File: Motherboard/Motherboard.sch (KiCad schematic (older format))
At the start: 116 parts, among them J1 Jack-DC_18v, J2 65SIB_Connector, J3 DB9_Header, J4 GPIO_Connector, J5 Expansion_Connector, J6 Expansion_Connector, J7 Expansion_Connector, J8 Expansion_Connector, J9 Expansion_Connector, P1 POWER TERMINAL, Q1 2N3055, Q2 TIC106, SW1 POWER SELECT, SW2 FUSE RESET, SW3 PROCESSOR RESET, U1 LM7812_TO220, U10 74HCT541, U11 28C256, U12 LM386, U13 LM7912_TO220, U14 74HCT00, U15 74HCT04, U16 74HCT574, U17 74HCT574, U18 74LS08, U19 28C256, U2 LM7805_TO220, U20 74LS138, U21 WD65C02, U22 74LS138, U23 74HCT04, U24 74HC74, U25 W65C51N, U26 NE555P, U27 WD65C22, U28 74LS138, U29 MAX235, U3 74LS08, U30 74LS138, U31 74HCT04, U32 74HCT04, U33 WD65C22, U34 74LS138, U35 74LS21, U36 74HCT04, U37 74LS21, U38 74HCT04, U39 74LS21, U4 74LS148, U40 74LS08, U41 74LS138, U42 74LS08, U43 74HCT04, U5 74LS85, U6 74HCT00, U7 74HCT04, U8 74LS08, U9 HM62256BLP, X1 ACO-8MHz, X2 ACO-1.8432MHz

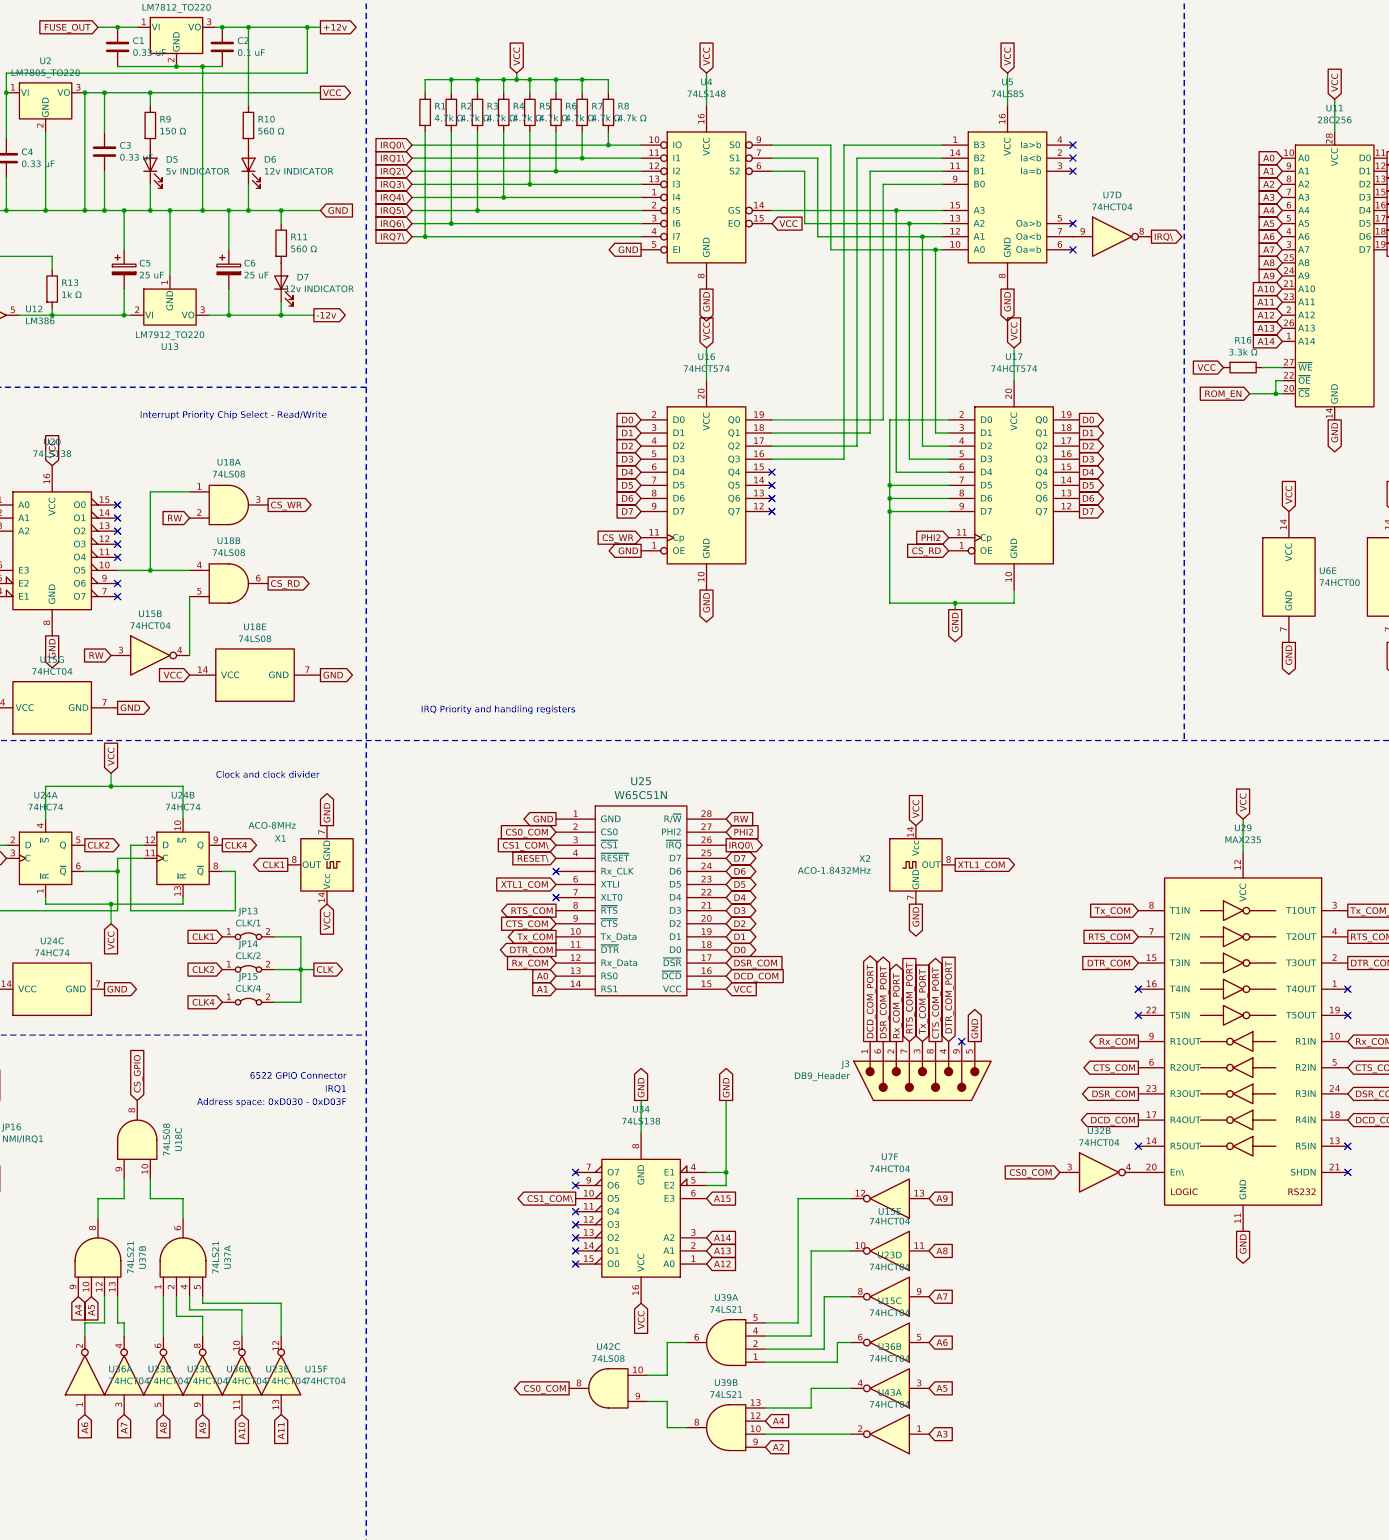
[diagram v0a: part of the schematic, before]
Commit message: Completed version 2 schematic...
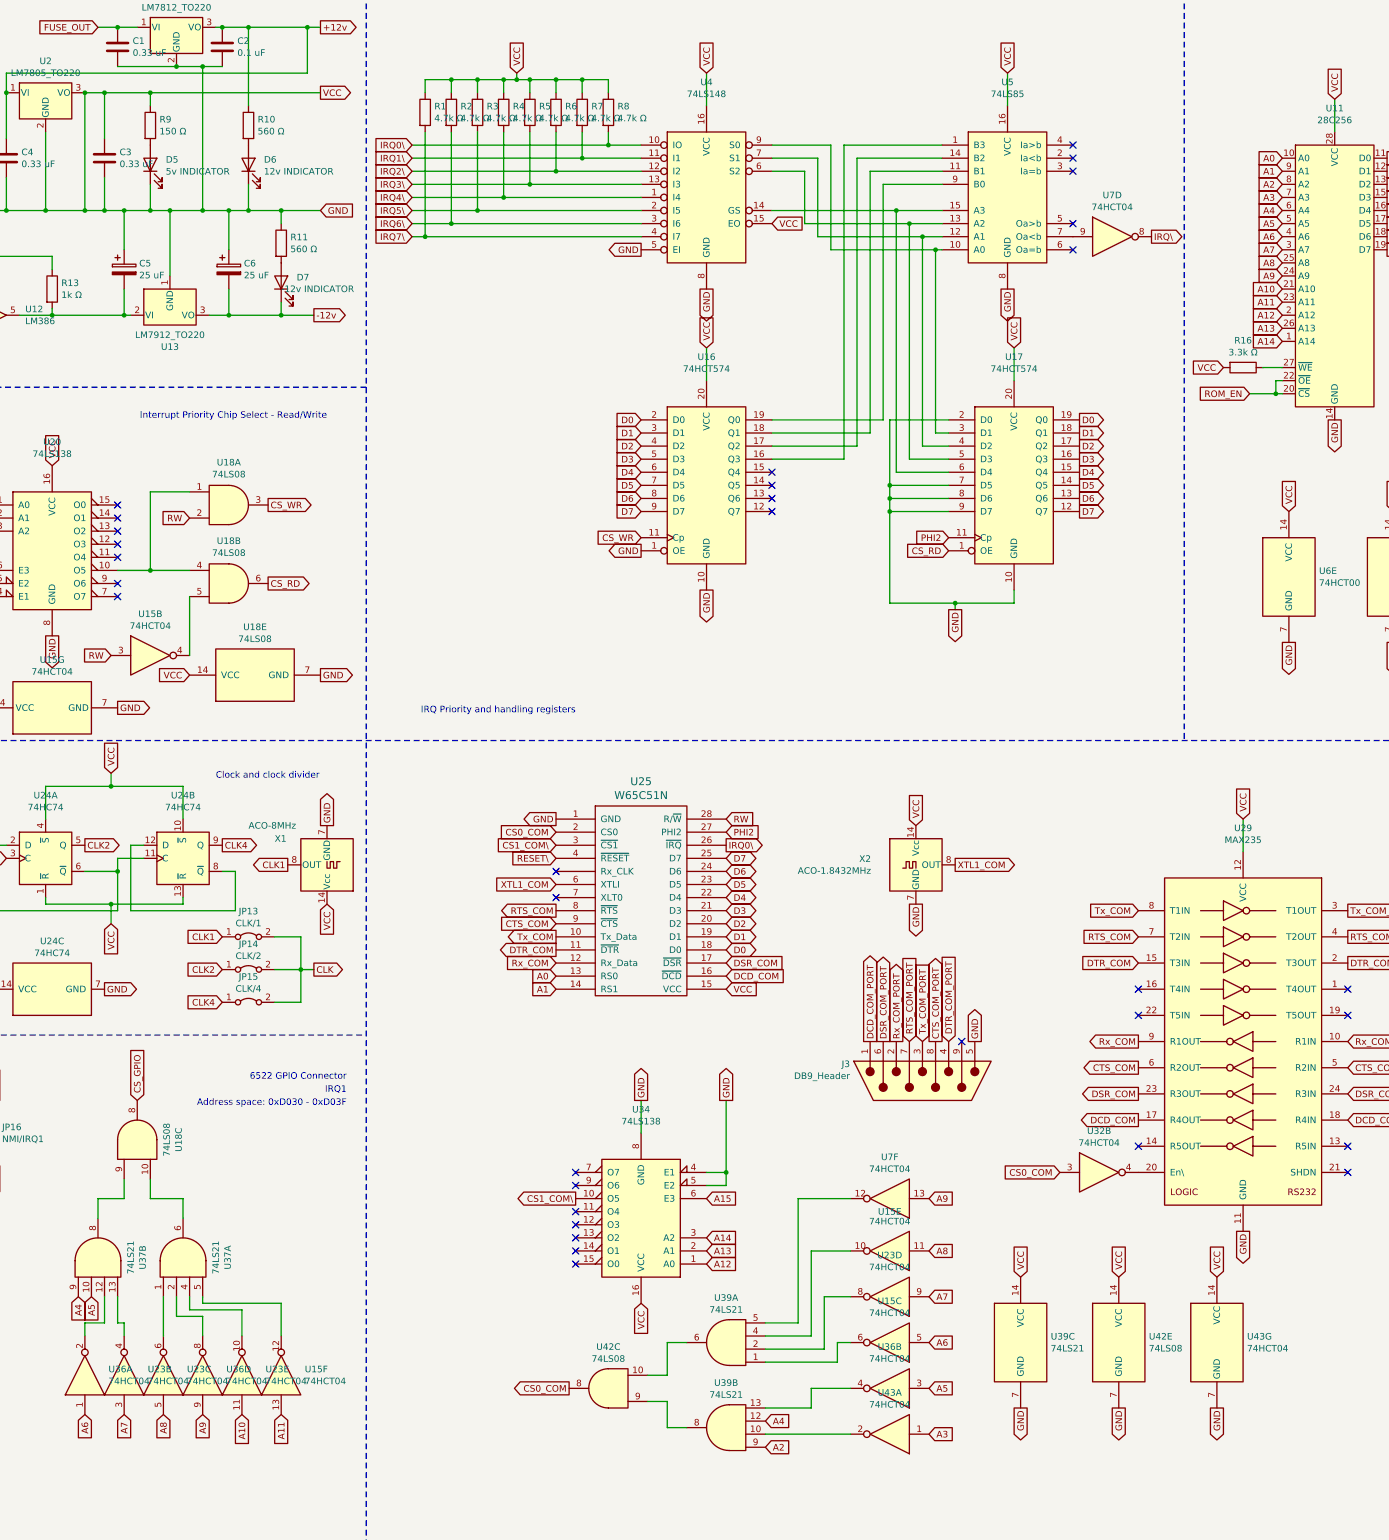
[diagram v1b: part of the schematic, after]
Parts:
- added unit 3 of U39
- added unit 5 of U42
- added unit 7 of U43
- U27: footprint Package_DIP:DIP-28_W15.24mm_Socket_LongPads -> Package_DIP:DIP-40_W15.24mm_Socket_LongPads
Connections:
- net GND: now also U39.14 (VCC), U39.7 (GND), U42.14 (VCC), U42.7 (GND), U43.14 (VCC), U43.7 (GND)
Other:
- moved on the sheet: C3
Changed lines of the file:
@@
 L Device:C C3
 U 1 1 61918BA3
-P 6700 2650
-F 0 "C3" H 6815 2696 50  0000 L CNN
-F 1 "0.33 uF" H 6815 2605 50  0000 L CNN
-F 2 "Capacitor_THT:C_Disc_D3.0mm_W1.6mm_P2.50mm" H 6738 2500 50  0001 C CNN
-F 3 "~" H 6700 2650 50  0001 C CNN
-	1    6700 2650
+P 6700 2700
+F 0 "C3" H 6815 2746 50  0000 L CNN
+F 1 "0.33 uF" H 6815 2655 50  0000 L CNN
+F 2 "Capacitor_THT:C_Disc_D3.0mm_W1.6mm_P2.50mm" H 6738 2550 50  0001 C CNN
+F 3 "~" H 6700 2700 50  0001 C CNN
+	1    6700 2700
 	1    0    0    -1
 $EndComp
 Wire Wire Line
-	6700 2800 6700 3100
-Wire Wire Line
-	6700 2500 6700 2200
-Wire Wire Line
 	2350 3100 3750 3100
 $Comp
@@
 Wire Wire Line
 	7050 2900 7050 3100
-Connection ~ 6700 3100
-Wire Wire Line
-	6700 2200 7050 2200
 Wire Wire Line
 	7050 2200 7050 2300
@@
 $EndComp
 Wire Wire Line
-	6550 2200 6700 2200
-Connection ~ 6700 2200
-Wire Wire Line
 	6250 2500 6250 3100
 $Comp
@@
 	7800 1700 8250 1700
 Connection ~ 6550 3100
-Wire Wire Line
-	6550 3100 6700 3100
 Connection ~ 6550 2200
 Wire Wire Line
@@
 $EndComp
 Wire Wire Line
-	6700 3100 6850 3100
-Wire Wire Line
 	7450 3100 7650 3100
 Wire Wire Line
@@
 F 0 "U27" H 24350 7413 60  0000 C CNN
 F 1 "WD65C22" H 24350 7519 60  0000 C CNN
-F 2 "Package_DIP:DIP-28_W15.24mm_Socket_LongPads" H 23850 8850 60  0001 C CNN
+F 2 "Package_DIP:DIP-40_W15.24mm_Socket_LongPads" H 23850 8850 60  0001 C CNN
 F 3 "" H 23850 8850 60  0000 C CNN
 	1    24350 8650
@@
 GND
 NoConn ~ 16200 10450
+$Comp
+L 74xx:74LS21 U39
+U 3 1 626DCCF3
+P 13700 11750
+F 0 "U39" H 13930 11796 50  0000 L CNN
+F 1 "74LS21" H 13930 11705 50  0000 L CNN
+F 2 "Package_DIP:DIP-14_W7.62mm_Socket_LongPads" H 13700 11750 50  0001 C CNN
+F 3 "http://www.ti.com/lit/gpn/sn74LS21" H 13700 11750 50  0001 C CNN
+	3    13700 11750
+	1    0    0    -1
+$EndComp
+Text GLabel 13700 11250 1    50   Input ~ 0
+VCC
+Text GLabel 13700 12250 3    50   Output ~ 0
+GND
+$Comp
+L 74xx:74LS08 U42
+U 5 1 626EAF96
+P 14450 11750
+F 0 "U42" H 14680 11796 50  0000 L CNN
+F 1 "74LS08" H 14680 11705 50  0000 L CNN
+F 2 "Package_DIP:DIP-14_W7.62mm_Socket_LongPads" H 14450 11750 50  0001 C CNN
+F 3 "http://www.ti.com/lit/gpn/sn74LS08" H 14450 11750 50  0001 C CNN
+	5    14450 11750
+	1    0    0    -1
+$EndComp
+Text GLabel 14450 11250 1    50   Input ~ 0
+VCC
+Text GLabel 14450 12250 3    50   Output ~ 0
+GND
+$Comp
+L 74xx:74HCT04 U43
+U 7 1 626F5FEB
+P 15200 11750
+F 0 "U43" H 15430 11796 50  0000 L CNN
+F 1 "74HCT04" H 15430 11705 50  0000 L CNN
+F 2 "Package_DIP:DIP-14_W7.62mm_Socket_LongPads" H 15200 11750 50  0001 C CNN
+F 3 "https://assets.nexperia.com/documents/data-sheet/74HC_HCT04.pdf" H 15200 11750 50  0001 C CNN
+	7    15200 11750
+	1    0    0    -1
+$EndComp
+Text GLabel 15200 11250 1    50   Input ~ 0
+VCC
+Text GLabel 15200 12250 3    50   Output ~ 0
+GND
+Wire Wire Line
+	6550 2200 6700 2200
+Wire Wire Line
+	6550 3100 6700 3100
+Wire Wire Line
+	6700 2850 6700 3100
+Connection ~ 6700 3100
+Wire Wire Line
+	6700 3100 6850 3100
+Wire Wire Line
+	6700 2550 6700 2200
+Connection ~ 6700 2200
+Wire Wire Line
+	6700 2200 7050 2200
 $EndSCHEMATC

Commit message: Various bug fixes and more traces added....
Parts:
- removed U20, U34, U41: 74LS138, Package_DIP:DIP-16_W7.62mm_Socket_LongPads, symbol 74xx:74LS138
- SW1: value POWER SELECT -> Barrel Jack / Mains
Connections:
- net 65SIB_CS2\ is gone; now on net DEV_CS\: U27.23 (~CS2), U28.10 (O5), U30.5 (E2)
- net CS1_COM\ is gone; now on net DEV_CS\: U25.3 (~CS1)
- net NMI\: no longer J5.28 (Pin_28), J6.28 (Pin_28), J7.28 (Pin_28), J8.28 (Pin_28), J9.28 (Pin_28)
- net DEV_CS\: now reaches U18.1, U18.4
- net DEV_CS\: now also U33.23 (~CS2)
- no-connect marks 68 -> 52
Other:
- moved on the sheet: U28
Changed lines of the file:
@@
 Wire Wire Line
 	2900 5650 3850 5650
-$Comp
-L 74xx:74LS138 U20
-U 1 1 6193D1D9
-P 6300 5650
-F 0 "U20" H 6300 6431 50  0000 C CNN
-F 1 "74LS138" H 6300 6340 50  0000 C CNN
-F 2 "Package_DIP:DIP-16_W7.62mm_Socket_LongPads" H 6300 5650 50  0001 C CNN
-F 3 "http://www.ti.com/lit/gpn/sn74LS138" H 6300 5650 50  0001 C CNN
-	1    6300 5650
-	1    0    0    -1
-$EndComp
-Text GLabel 5800 5350 0    50   Input ~ 0
-A12
-Text GLabel 5800 5450 0    50   Input ~ 0
-A13
-Text GLabel 5800 5550 0    50   Input ~ 0
-A14
-Text GLabel 5800 5850 0    50   Input ~ 0
-A15
-Text GLabel 6300 6350 3    50   Output ~ 0
-GND
-Text GLabel 5800 5950 0    50   Output ~ 0
-GND
-Text GLabel 5800 6050 0    50   Output ~ 0
-GND
 Text GLabel 6750 6500 0    50   Input ~ 0
 RW
 Wire Wire Line
-	6800 5850 7050 5850
-Wire Wire Line
 	7350 5250 7050 5250
 Wire Wire Line
-	7050 5250 7050 5850
-Connection ~ 7050 5850
+	7050 5250 7050 5550
 Wire Wire Line
 	7050 5850 7350 5850
@@
 Text GLabel 7950 5950 2    50   Output ~ 0
 CS_RD
-NoConn ~ 6800 5350
-NoConn ~ 6800 5450
-NoConn ~ 6800 5550
-NoConn ~ 6800 5650
-NoConn ~ 6800 5750
-NoConn ~ 6800 5950
-NoConn ~ 6800 6050
 $Comp
 L Timer:NE555P U26
@@
 Text GLabel 2350 9850 0    50   Output ~ 0
 GND
-$Comp
-L 74xx:74LS138 U41
-U 1 1 61AADD06
-P 5150 12050
-F 0 "U41" H 5150 11169 50  0000 C CNN
-F 1 "74LS138" H 5150 11260 50  0000 C CNN
-F 2 "Package_DIP:DIP-16_W7.62mm_Socket_LongPads" H 5150 12050 50  0001 C CNN
-F 3 "http://www.ti.com/lit/gpn/sn74LS138" H 5150 12050 50  0001 C CNN
-	1    5150 12050
-	-1   0    0    1
-$EndComp
-Wire Wire Line
-	5650 11650 5750 11650
-Wire Wire Line
-	5750 11650 5750 11350
-Wire Wire Line
-	5650 11750 5750 11750
-Wire Wire Line
-	5750 11750 5750 11650
-Connection ~ 5750 11650
-Text GLabel 5650 11850 2    50   Input ~ 0
-A15
-Text GLabel 5650 12150 2    50   Input ~ 0
-A14
-Text GLabel 5650 12250 2    50   Input ~ 0
-A13
-Text GLabel 5650 12350 2    50   Input ~ 0
-A12
-Text GLabel 5150 12650 3    50   Input ~ 0
-VCC
-Text GLabel 5150 11150 1    50   Output ~ 0
-GND
-Text GLabel 5750 11350 1    50   Output ~ 0
-GND
 Text GLabel 6950 9900 1    50   Input ~ 0
 CS_GPIO
@@
 Text GLabel 13600 3700 3    50   Output ~ 0
 GND
-NoConn ~ 4650 11650
-NoConn ~ 4650 11750
-NoConn ~ 4650 11950
-NoConn ~ 4650 12050
-NoConn ~ 4650 12150
-NoConn ~ 4650 12250
-NoConn ~ 4650 12350
 Text GLabel 3650 11750 2    50   Output ~ 0
 IRQ_DECIDE\
-Wire Wire Line
-	4250 11850 4250 11550
-Wire Wire Line
-	3650 11550 4250 11550
-Wire Wire Line
-	4650 11850 4250 11850
 $Comp
 L PC_Jumpers:Jumper_3_Bridged12 JP16
@@
 Text GLabel 5850 10400 3    50   Output ~ 0
 NMI\
-$Comp
-L 74xx:74LS138 U34
-U 1 1 61D4A52C
-P 10800 10850
-F 0 "U34" H 10800 9969 50  0000 C CNN
-F 1 "74LS138" H 10800 10060 50  0000 C CNN
-F 2 "Package_DIP:DIP-16_W7.62mm_Socket_LongPads" H 10800 10850 50  0001 C CNN
-F 3 "http://www.ti.com/lit/gpn/sn74LS138" H 10800 10850 50  0001 C CNN
-	1    10800 10850
-	-1   0    0    1
-$EndComp
 Text GLabel 13350 9450 1    50   Output ~ 0
 GND
@@
 Wire Wire Line
 	11000 12000 10850 12000
-Text GLabel 11300 10650 2    50   Input ~ 0
-A15
-Text GLabel 11300 10950 2    50   Input ~ 0
-A14
-Text GLabel 11300 11050 2    50   Input ~ 0
-A13
-Text GLabel 11300 11150 2    50   Input ~ 0
-A12
 Text GLabel 10250 12100 0    50   Output ~ 0
 CS0_COM
@@
 	0    1    1    0
 $EndComp
-Wire Wire Line
-	10800 10150 10800 9900
-NoConn ~ 10300 10950
-NoConn ~ 10300 11050
-NoConn ~ 10300 11150
-NoConn ~ 10300 10850
-NoConn ~ 10300 10750
-NoConn ~ 10300 10550
-NoConn ~ 10300 10450
-Wire Wire Line
-	11450 10450 11450 10550
-Connection ~ 11450 10450
-Wire Wire Line
-	11450 9900 11450 10450
-Wire Wire Line
-	11300 10550 11450 10550
-Wire Wire Line
-	11300 10450 11450 10450
-Text GLabel 11450 9900 1    50   Output ~ 0
-GND
-Text GLabel 10800 9900 1    50   Output ~ 0
-GND
-Text GLabel 10800 11450 3    50   Input ~ 0
-VCC
 Text GLabel 10150 7750 0    50   Output ~ 0
 GND
@@
 P 5250 2200
 F 0 "SW1" H 5250 1875 50  0000 C CNN
-F 1 "POWER SELECT" H 5250 1966 50  0000 C CNN
+F 1 "Barrel Jack / Mains" H 5250 1966 50  0000 C CNN
 F 2 "Button_Switch_THT:SW_Slide_1P2T_CK_OS102011MS2Q" H 5250 2200 50  0001 C CNN
 F 3 "~" H 5250 2200 50  0001 C CNN
@@
 65SIB_CS3
 Text GLabel 26300 9650 0    50   Input ~ 0
-65SIB_CS2\
+DEV_CS\
 Text GLabel 23700 7850 0    50   Input ~ 0
-65SIB_CS2\
+DEV_CS\
 Text GLabel 23700 7950 0    50   Input ~ 0
 65SIB_CS3
@@
 L 74xx:74LS138 U28
 U 1 1 6E11B869
-P 20350 9100
-F 0 "U28" H 20350 9881 50  0000 C CNN
-F 1 "74LS138" H 20350 9790 50  0000 C CNN
-F 2 "Package_DIP:DIP-16_W7.62mm_Socket_LongPads" H 20350 9100 50  0001 C CNN
-F 3 "http://www.ti.com/lit/gpn/sn74LS138" H 20350 9100 50  0001 C CNN
-	1    20350 9100
+P 20150 9100
+F 0 "U28" H 20150 9881 50  0000 C CNN
+F 1 "74LS138" H 20150 9790 50  0000 C CNN
+F 2 "Package_DIP:DIP-16_W7.62mm_Socket_LongPads" H 20150 9100 50  0001 C CNN
+F 3 "http://www.ti.com/lit/gpn/sn74LS138" H 20150 9100 50  0001 C CNN
+	1    20150 9100
 	1    0    0    -1
 $EndComp
-Text GLabel 19850 8800 0    50   Input ~ 0
+Text GLabel 19650 8800 0    50   Input ~ 0
 A12
-Text GLabel 19850 8900 0    50   Input ~ 0
+Text GLabel 19650 8900 0    50   Input ~ 0
 A13
-Text GLabel 19850 9000 0    50   Input ~ 0
+Text GLabel 19650 9000 0    50   Input ~ 0
 A14
-Text GLabel 19850 9300 0    50   Input ~ 0
+Text GLabel 19650 9300 0    50   Input ~ 0
 A15
-Text GLabel 20850 9300 2    50   Output ~ 0
-65SIB_CS2\
-Text GLabel 19850 9400 0    50   Output ~ 0
-GND
-Text GLabel 19850 9500 0    50   Output ~ 0
-GND
-NoConn ~ 20850 8800
-NoConn ~ 20850 8900
-NoConn ~ 20850 9000
-NoConn ~ 20850 9100
-NoConn ~ 20850 9200
-NoConn ~ 20850 9400
-NoConn ~ 20850 9500
-Text GLabel 20350 8250 1    50   Input ~ 0
+Text GLabel 20650 9300 2    50   Output ~ 0
+DEV_CS\
+Text GLabel 19650 9400 0    50   Output ~ 0
+GND
+Text GLabel 19650 9500 0    50   Output ~ 0
+GND
+NoConn ~ 20650 8800
+NoConn ~ 20650 8900
+NoConn ~ 20650 9000
+NoConn ~ 20650 9100
+NoConn ~ 20650 9200
+NoConn ~ 20650 9400
+NoConn ~ 20650 9500
+Text GLabel 20150 8250 1    50   Input ~ 0
 VCC
 Wire Wire Line
-	20350 8250 20350 8500
+	20150 8250 20150 8500
 $Comp
 L Graphic:SYM_Flash_XLarge #SYM1
@@
 Text GLabel 23750 12700 2    50   Output ~ 0
 IRQ3\
-Text GLabel 23750 12600 2    50   Output ~ 0
-NMI\
 Text GLabel 23750 12500 2    50   Output ~ 0
 Page_En
@@
 Text GLabel 25400 12700 2    50   Output ~ 0
 IRQ3\
-Text GLabel 25400 12600 2    50   Output ~ 0
-NMI\
 Text GLabel 25400 12500 2    50   Output ~ 0
 Page_En
@@
 Text GLabel 27000 12700 2    50   Output ~ 0
 IRQ3\
-Text GLabel 27000 12600 2    50   Output ~ 0
-NMI\
 Text GLabel 27000 12500 2    50   Output ~ 0
 Page_En
@@
 Text GLabel 28600 12700 2    50   Output ~ 0
 IRQ3\
-Text GLabel 28600 12600 2    50   Output ~ 0
-NMI\
 Text GLabel 28600 12500 2    50   Output ~ 0
 Page_En
@@
 Text GLabel 30150 12700 2    50   Output ~ 0
 IRQ3\
-Text GLabel 30150 12600 2    50   Output ~ 0
-NMI\
 Text GLabel 30150 12500 2    50   Output ~ 0
 Page_En
@@
 Text GLabel 29650 11300 0    50   Input ~ 0
 VCC
-Text GLabel 20350 9800 3    50   Output ~ 0
+Text GLabel 20150 9800 3    50   Output ~ 0
 GND
 Text GLabel 23700 9350 0    50   Input ~ 0
@@
 Connection ~ 5950 2200
 Text GLabel 10150 7950 0    50   Input ~ 0
-CS1_COM\
-Text GLabel 10300 10650 0    50   Output ~ 0
-CS1_COM\
+DEV_CS\
 $Comp
 L 74xx:74HCT04 U32
@@
 Text GLabel 14000 10450 0    50   Input ~ 0
 CS0_COM
-Text GLabel 6300 5050 1    50   Input ~ 0
-VCC
 $Comp
 L 74xx:74LS08 U18
@@
 Text GLabel 4800 9900 2    50   Output ~ 0
 GND
-Wire Wire Line
-	5150 11150 5150 11350
 NoConn ~ 10150 8350
 $Comp
@@
 Wire Wire Line
 	6700 2200 7050 2200
+NoConn ~ 30150 12600
+NoConn ~ 28600 12600
+NoConn ~ 27000 12600
+NoConn ~ 25400 12600
+NoConn ~ 23750 12600
+Text GLabel 3650 11550 2    50   Input ~ 0
+DEV_CS\
+Wire Wire Line
+	7050 5550 7000 5550
+Connection ~ 7050 5550
+Wire Wire Line
+	7050 5550 7050 5850
+Text GLabel 7000 5550 0    50   Input ~ 0
+DEV_CS\
 $EndSCHEMATC
